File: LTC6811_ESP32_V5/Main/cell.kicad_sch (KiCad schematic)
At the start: 6 parts, among them Q22 TSM2323

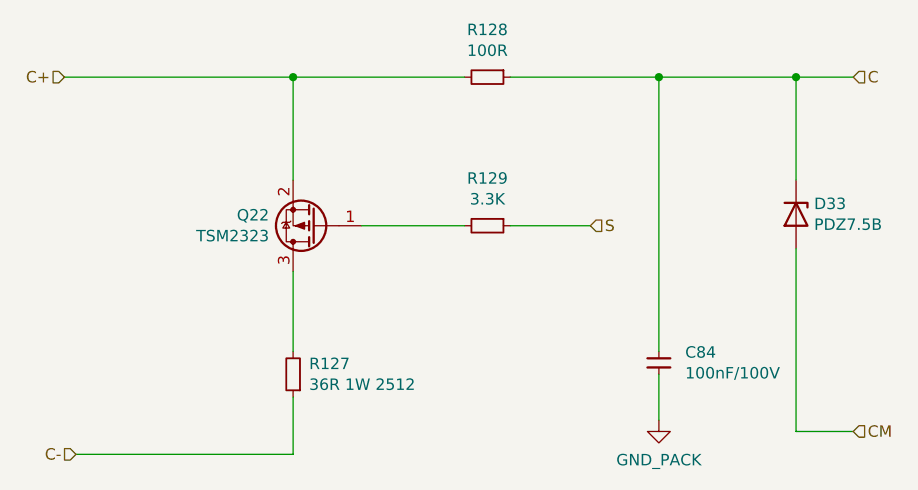
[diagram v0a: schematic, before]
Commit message: fix page number
fix page number
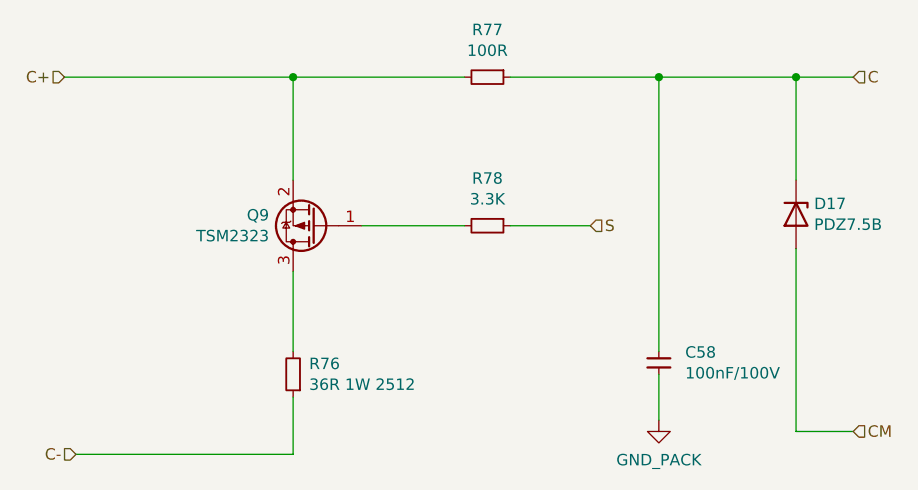
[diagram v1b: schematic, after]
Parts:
- renumbered C84 to C58, D33 to D17, Q22 to Q9, R127 to R76, R128 to R77, R129 to R78
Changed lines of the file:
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@@
 		(on_board yes)
 		(dnp no)
-		(property "Reference" "Q22"
+		(property "Reference" "Q9"
 			(at 64.008 47.7266 0)
 			(effects
@@
 		(dnp no)
 		(fields_autoplaced yes)
-		(property "Reference" "#PWR099"
+		(property "Reference" "#PWR072"
 			(at 107.315 76.835 0)
 			(effects
@@
 		(on_board yes)
 		(dnp no)
-		(property "Reference" "R129"
+		(property "Reference" "R78"
 			(at 88.265 43.6372 90)
 			(effects
@@
 		(on_board yes)
 		(dnp no)
-		(property "Reference" "C84"
+		(property "Reference" "C58"
 			(at 110.236 62.9666 0)
 			(effects
@@
 		(on_board yes)
 		(dnp no)
-		(property "Reference" "R127"
+		(property "Reference" "R76"
 			(at 68.453 64.2366 0)
 			(effects
@@
 		(on_board yes)
 		(dnp no)
-		(property "Reference" "D33"
+		(property "Reference" "D17"
 			(at 124.5616 46.4566 90)
 			(effects
@@
 		(on_board yes)
 		(dnp no)
-		(property "Reference" "R128"
+		(property "Reference" "R77"
 			(at 88.265 27.1272 90)
 			(effects

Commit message: Add files via upload
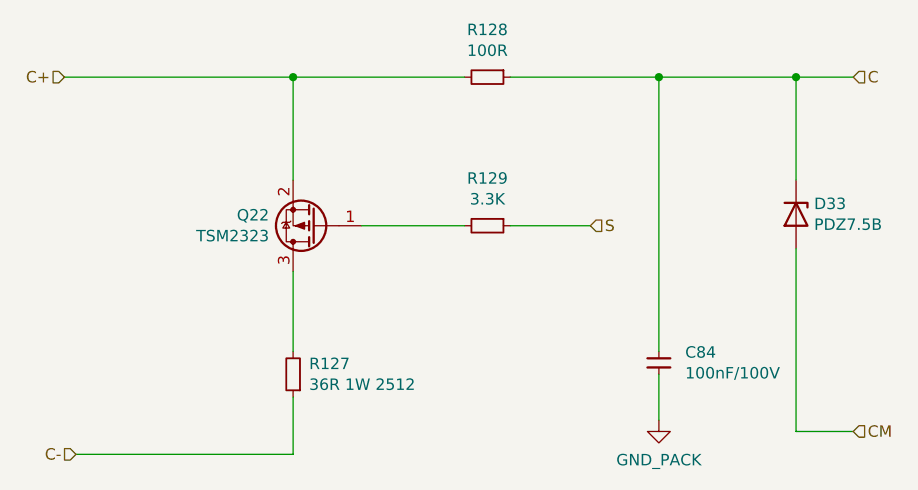
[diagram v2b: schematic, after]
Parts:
- renumbered C58 to C84, D17 to D33, Q9 to Q22, R76 to R127, R77 to R128, R78 to R129
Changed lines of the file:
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@@
 		(on_board yes)
 		(dnp no)
-		(property "Reference" "Q9"
+		(property "Reference" "Q22"
 			(at 64.008 47.7266 0)
 			(effects
@@
 		(dnp no)
 		(fields_autoplaced yes)
-		(property "Reference" "#PWR072"
+		(property "Reference" "#PWR099"
 			(at 107.315 76.835 0)
 			(effects
@@
 		(on_board yes)
 		(dnp no)
-		(property "Reference" "R78"
+		(property "Reference" "R129"
 			(at 88.265 43.6372 90)
 			(effects
@@
 		(on_board yes)
 		(dnp no)
-		(property "Reference" "C58"
+		(property "Reference" "C84"
 			(at 110.236 62.9666 0)
 			(effects
@@
 		(on_board yes)
 		(dnp no)
-		(property "Reference" "R76"
+		(property "Reference" "R127"
 			(at 68.453 64.2366 0)
 			(effects
@@
 		(on_board yes)
 		(dnp no)
-		(property "Reference" "D17"
+		(property "Reference" "D33"
 			(at 124.5616 46.4566 90)
 			(effects
@@
 		(on_board yes)
 		(dnp no)
-		(property "Reference" "R77"
+		(property "Reference" "R128"
 			(at 88.265 27.1272 90)
 			(effects
